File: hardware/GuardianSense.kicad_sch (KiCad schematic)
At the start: 41 parts, among them J1 Conn_01x03_Pin AM312 Module, J2 Micro_SD_Card, P1 USB_C_Plug_USB2.0, Q1 BC847, SW1 SW_SPST, SW2 SW_SPST, U1 ESP32-S3-WROOM-1, U2 D3V3XA4B10LP, U3 AMS1117-3.3, U4 BME280

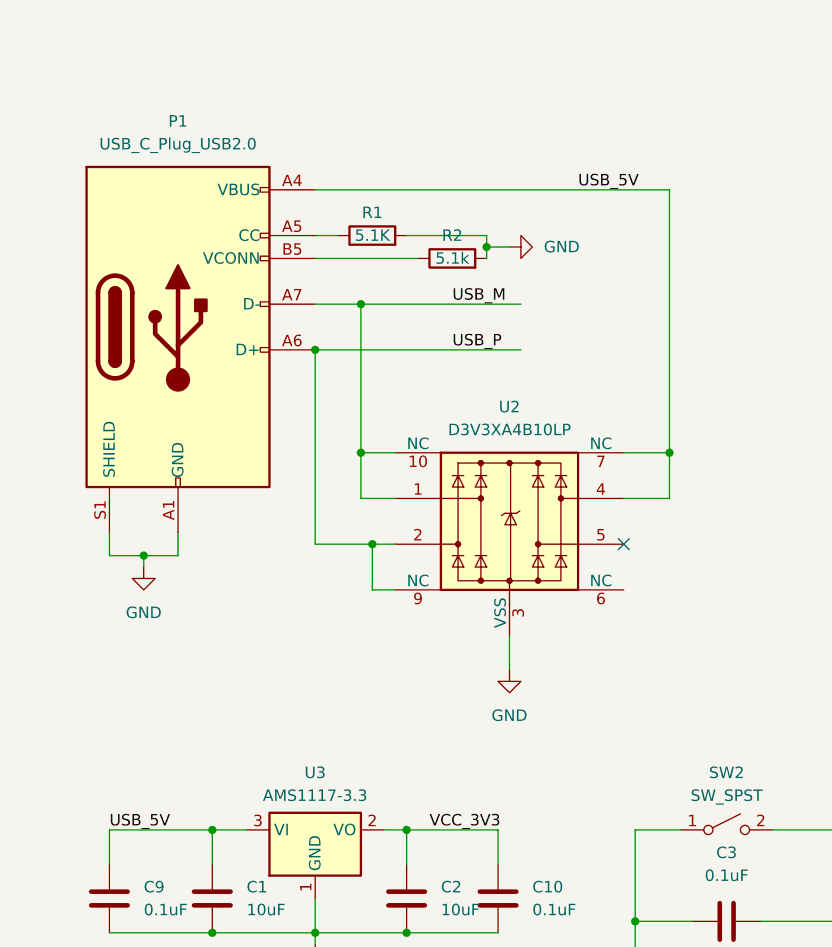
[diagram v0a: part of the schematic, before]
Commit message: Updates
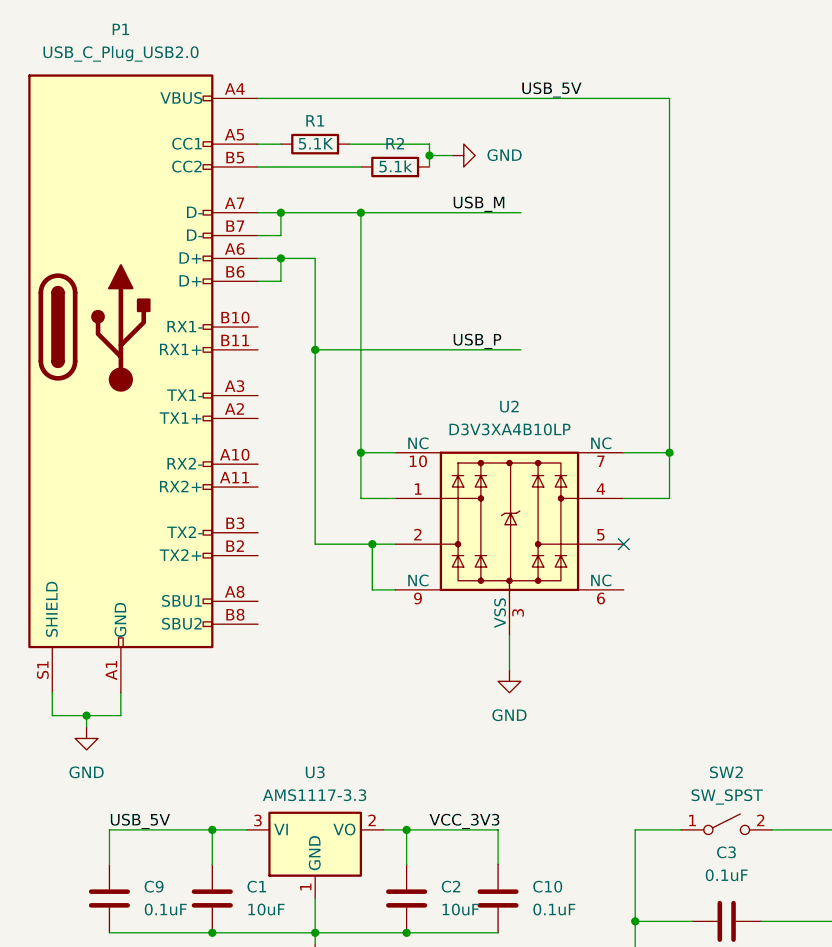
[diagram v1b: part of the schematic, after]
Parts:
- P1: symbol Connector:USB_C_Plug_USB2.0 -> Connector:USB_C_Receptacle
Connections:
- net USB_M: now also P1.B7 (D-)
- net USB_P: now also P1.B6 (D+)
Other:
- moved on the sheet: R1, R2
